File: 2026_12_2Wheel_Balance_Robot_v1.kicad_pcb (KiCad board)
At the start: 2 copper layers, 73.5 x 74.5 mm, 56 parts, among them J1 Conn_01x04, J2 CONN_MPU6050, J3 USB_C_Receptacle_USB2.0_14P, J4 ESP_Conn, J5 BATT_CONN, J6 M1_CONN, J7 M2_CONN, J8 ENCODER_CONN, J9 MT6701_CONN, SW2 SW_uP_Reset, U1 STM32F401RBTx, U2 TB6612FNG, U3 LD1117S50TR_SOT223, U5 USBLC6-2SC6, U6 LD1117S33TR_SOT223, Y3 16MHz

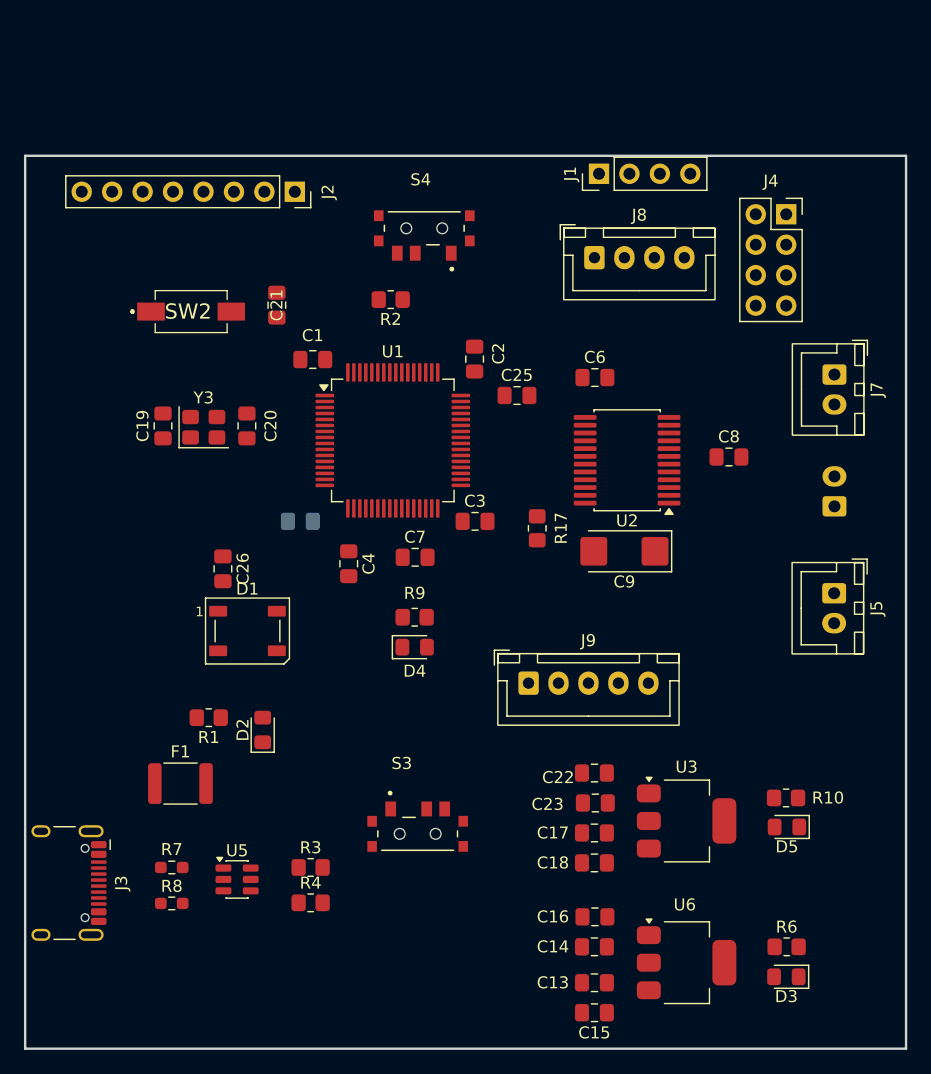
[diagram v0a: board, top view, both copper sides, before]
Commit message: homework push
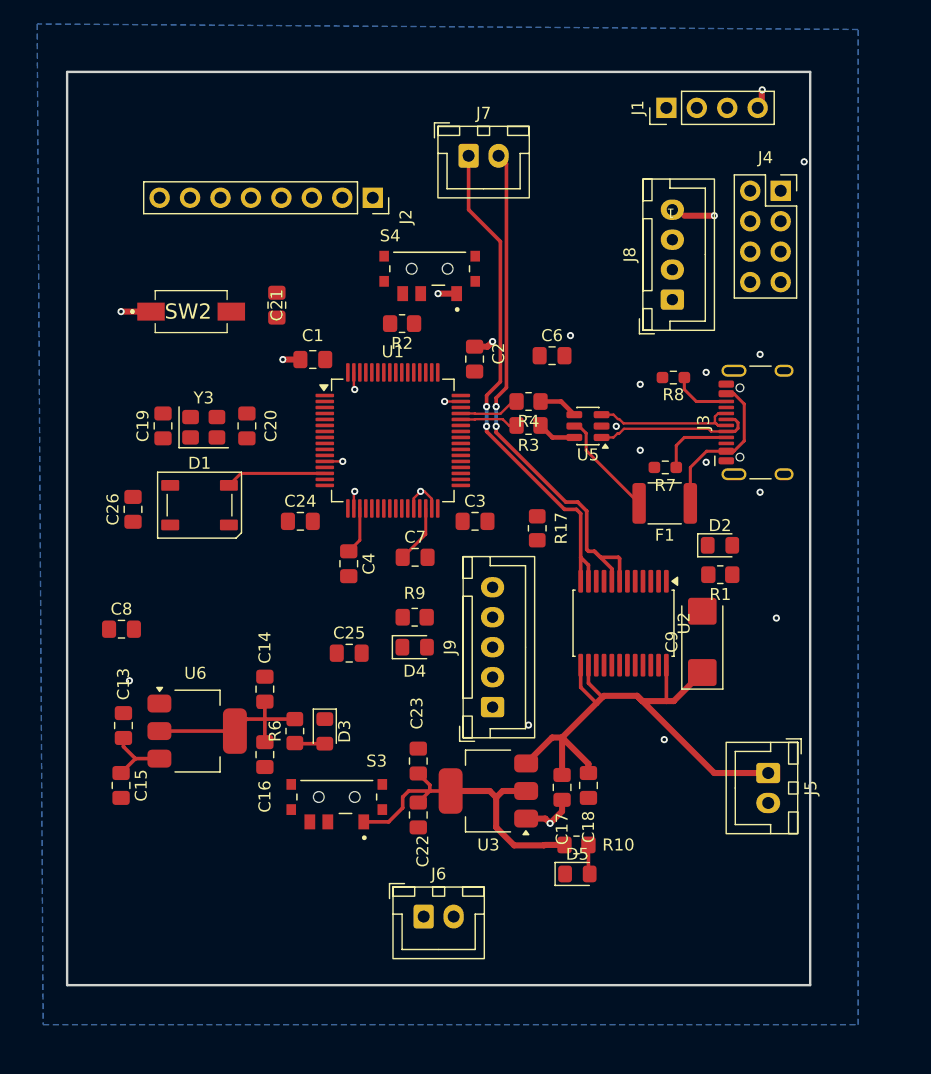
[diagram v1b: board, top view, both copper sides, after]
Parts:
- C24, J6: moved to F.Cu
- moved J3 71.1 mm to (153.7, 82.2), turned to 90 degrees
- moved R8 60.6 mm to (145.6, 78.5), turned to 180 degrees
- moved R7 53.0 mm to (144.9, 86.0), turned to 0 degrees
- moved C8 52.7 mm to (99.5, 99.5)
- moved J6 48.4 mm to (124.8, 123.5), turned to 0 degrees
- moved U5 47.8 mm to (138.5, 82.5), turned to 180 degrees
- moved F1 46.7 mm to (144.9, 89.0), turned to 180 degrees
- moved R4 45.6 mm to (133.5, 80.5), turned to 180 degrees
- moved U6 45.2 mm to (105.8, 108.0)
- moved R6 44.8 mm to (114.0, 108.0), turned to 90 degrees
- moved C13 44.8 mm to (99.7, 107.5), turned to 90 degrees
- moved R1 44.3 mm to (149.5, 95.0)
- moved C15 43.8 mm to (99.5, 112.5), turned to -90 degrees
- moved D3 43.6 mm to (116.5, 108.0), turned to -90 degrees
- moved D2 41.1 mm to (149.5, 92.5), turned to 0 degrees
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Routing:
- net VM: track 0.00 -> 48.7 mm
- net /MD_BO2: track 0.00 -> 45.3 mm, vias 0 -> 2
- net /MD_BO1: track 0.00 -> 43.2 mm, vias 0 -> 2
- net 5V_REG: track 0.00 -> 27.7 mm
- net GND: track 0.00 -> 23.6 mm, vias 0 -> 25
- net +3.3V: track 0.00 -> 19.6 mm
- net /USB_D-: track 0.00 -> 13.5 mm
- net Net-(F1-~-Pad1): track 0.00 -> 13.3 mm
- net /USB_D+: track 0.00 -> 12.7 mm
- net Vusb: track 0.00 -> 8.92 mm
- net /WS_DIN: track 0.00 -> 8.41 mm
- net Net-(J3-CC1): track 0.00 -> 6.28 mm
- net +5V: track 0.00 -> 5.84 mm
- net /ESD_D+: track 0.00 -> 5.08 mm
- net Net-(J3-CC2): track 0.00 -> 4.91 mm
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- added copper zone on B.Cu, net GND
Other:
- board size 73.5 x 74.5 mm -> 62 x 76.2 mm
